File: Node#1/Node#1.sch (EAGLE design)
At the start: 197 parts, among them J1 1757242, J2 DCJ200-10-A-XX-X_REVA, K1 FTR-K1CK005W, K2 FTR-K1CK005W, K3 FTR-K1CK005W, K4 FTR-K1CK005W, U10 ULN2003AIDG4, U11 BLUENRG-232, U12 ACS723LLCTR-40AB-T, U13 RV8564C3, U14 ACS723LLCTR-40AB-T, U2 SEMTECH_SX1503I091TRTSEMTECH_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, U3 MIC4468YWM, U4 LM339ADR, U5 74HC08D,652, U6 SN74LVC1G74DCUR, U7 TMP75BID, U8 IRM-05-5, U9 LMS8117AMP-3.3, X1 2081-1228, X2 2081-1228, X3 2081-1228, X4 2081-1222, Y3 ECS-160-12-36-AGN-TR, Y4 NX2012SA-32.768K-STD-MUB-1

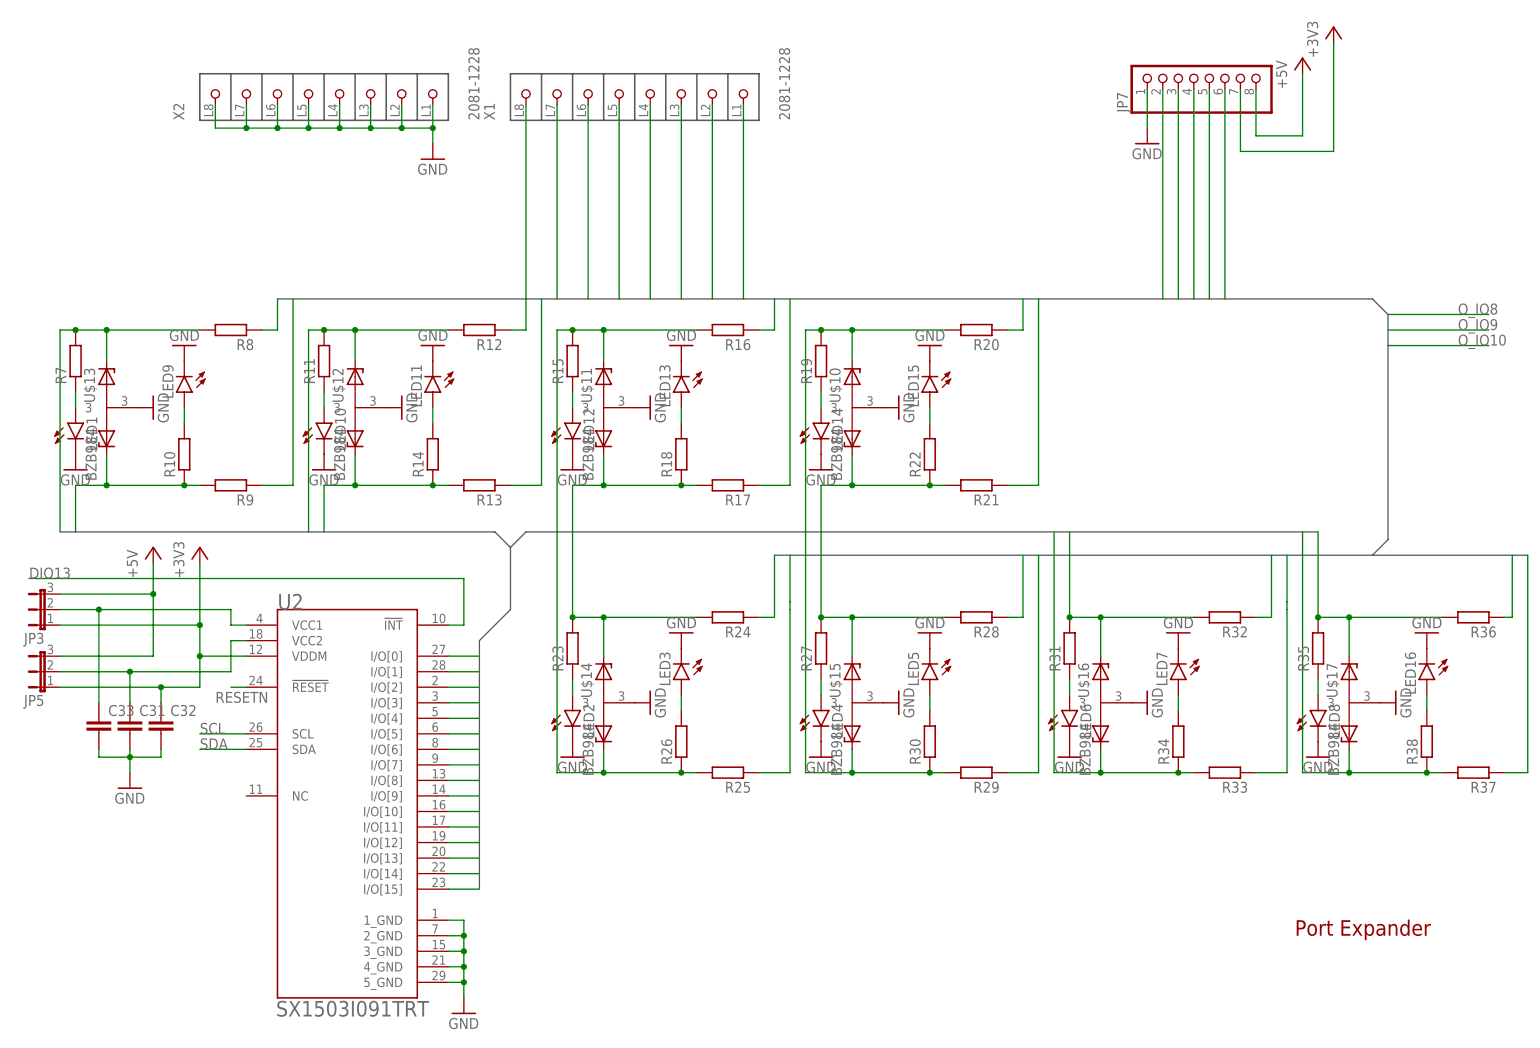
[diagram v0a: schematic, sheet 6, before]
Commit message: Redone Node#1 Layout
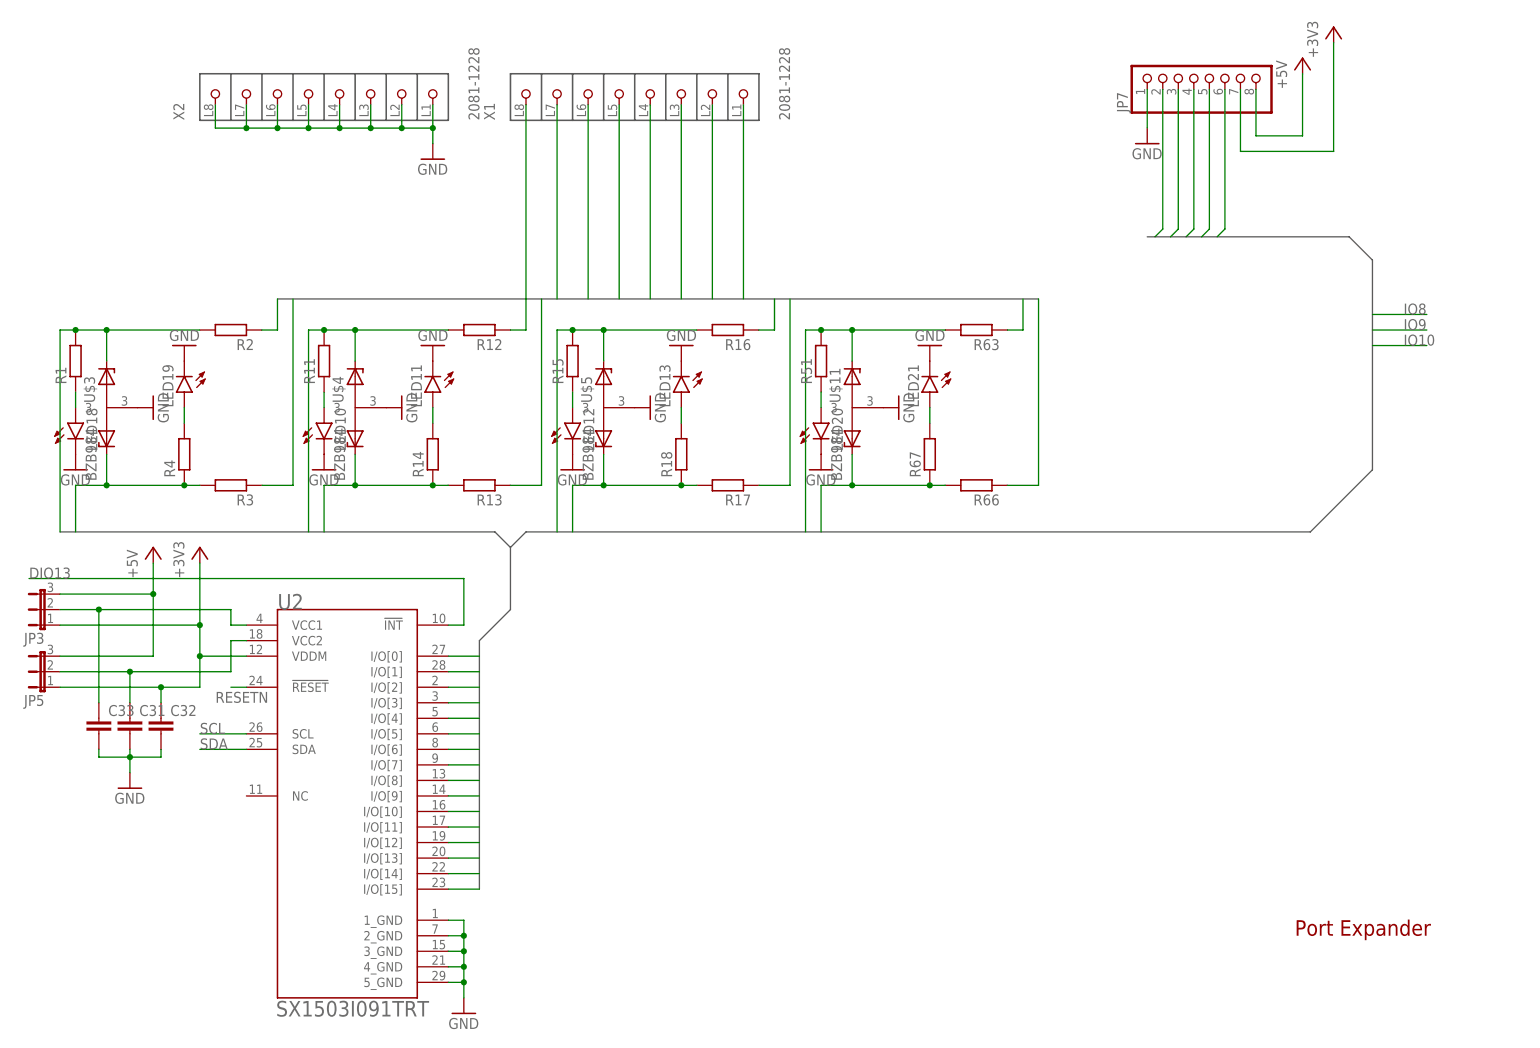
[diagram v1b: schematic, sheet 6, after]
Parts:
- removed LED16, LED2, LED3, LED4, LED5, LED6, LED7, LED8: (no value), led:LED3MM
- removed R23, R24, R25, R26, R27, R28, R29, R30, R31, R32, R33, R34, R35, R36, R37, R38: (no value), rcl:R-EU_R0805
- removed U$10, U$14, U$15, U$16, U$17: BZB984, BlueHome:BZB984
- added U$5: BZB984, BlueHome:BZB984
- renumbered LED1 to LED18, LED14 to LED20, LED15 to LED21, LED9 to LED19, R10 to R4, R19 to R51, R20 to R63, R21 to R66, R22 to R67, R7 to R1, R8 to R2, R9 to R3, U$12 to U$4, U$13 to U$3
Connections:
- removed net E_SHORT: U5.4B, U6.Q
- removed net E_TEMP: R50.1, U5.4A, U7.ALERT
- removed net N$54: LED2.A, R23.1
- removed net N$58: LED3.A, R26.2
- removed net N$60: LED4.A, R27.1
- removed net N$62: LED5.A, R30.2
- removed net N$64: LED6.A, R31.1
- removed net N$66: LED7.A, R34.2
- removed net N$69: LED8.A, R35.1
- removed net N$72: LED16.A, R38.2
- removed net O_IO10: R28.1
- removed net O_IO11: JP7.2, R29.1, R32.1
- removed net O_IO12: JP7.3, R33.1
- removed net O_IO13: JP7.4, R36.1
- removed net O_IO14: JP7.5, R37.1
- removed net O_IO15: JP7.6
- removed net O_IO8: R24.1
- removed net O_IO9: R25.1
- net ERROR: no longer R49.1, U5.4Y
- net GND: now also U$5.3; no longer LED16.C, LED2.C, LED3.C, LED4.C, LED5.C, LED6.C, LED7.C, LED8.C, U$10.3, U$14.3, U$15.3, U$16.3, U$17.3
- net IO10: now also R50.1, U5.4A, U7.ALERT; no longer R27.2, R28.2, U$15.1
- net IO11: now also JP7.2; no longer R29.2, R30.1, U$15.2
- net IO12: now also JP7.3; no longer R31.2, R32.2, U$16.1
- net IO13: now also JP7.4; no longer R33.2, R34.1, U$16.2
- net IO14: now also JP7.5; no longer R35.2, R36.2, U$17.1
- net IO15: now also JP7.6; no longer R37.2, R38.1, U$17.2
- net IO4: now also U$5.1; no longer U$11.1
- net IO5: now also U$5.2; no longer U$11.2
- net IO6: now also U$11.1; no longer U$10.1
- net IO7: now also U$11.2; no longer U$10.2
- net IO8: now also R49.1, U5.4Y; no longer R23.2, R24.2, U$14.1
- net IO9: now also U5.4B, U6.Q; no longer R25.2, R26.1, U$14.2
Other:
- moved on the sheet: U$11

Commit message: Arrangement of Node#1 - DC Power Jack
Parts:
- R53: device rcl:R-EU_R1210 -> rcl:R-EU_R0805
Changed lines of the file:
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@@
 <grid distance="0.1" unitdist="inch" unit="inch" style="lines" multiple="1" display="no" altdistance="0.01" altunitdist="inch" altunit="inch"/>
 <layers>
-<layer number="1" name="Top" color="4" fill="1" visible="no" active="no"/>
-<layer number="2" name="Route2" color="16" fill="1" visible="no" active="no"/>
-<layer number="3" name="Route3" color="17" fill="1" visible="no" active="no"/>
-<layer number="4" name="Route4" color="18" fill="1" visible="no" active="no"/>
-<layer number="5" name="Route5" color="19" fill="1" visible="no" active="no"/>
-<layer number="6" name="Route6" color="25" fill="1" visible="no" active="no"/>
-<layer number="7" name="Route7" color="26" fill="1" visible="no" active="no"/>
-<layer number="8" name="Route8" color="27" fill="1" visible="no" active="no"/>
-<layer number="9" name="Route9" color="28" fill="1" visible="no" active="no"/>
-<layer number="10" name="Route10" color="29" fill="1" visible="no" active="no"/>
-<layer number="11" name="Route11" color="30" fill="1" visible="no" active="no"/>
-<layer number="12" name="Route12" color="20" fill="1" visible="no" active="no"/>
-<layer number="13" name="Route13" color="21" fill="1" visible="no" active="no"/>
-<layer number="14" name="Route14" color="22" fill="1" visible="no" active="no"/>
-<layer number="15" name="Route15" color="23" fill="1" visible="no" active="no"/>
-<layer number="16" name="Bottom" color="1" fill="1" visible="no" active="no"/>
-<layer number="17" name="Pads" color="2" fill="1" visible="no" active="no"/>
-<layer number="18" name="Vias" color="2" fill="1" visible="no" active="no"/>
-<layer number="19" name="Unrouted" color="6" fill="1" visible="no" active="no"/>
-<layer number="20" name="Dimension" color="24" fill="1" visible="no" active="no"/>
-<layer number="21" name="tPlace" color="7" fill="1" visible="no" active="no"/>
-<layer number="22" name="bPlace" color="7" fill="1" visible="no" active="no"/>
-<layer number="23" name="tOrigins" color="15" fill="1" visible="no" active="no"/>
-<layer number="24" name="bOrigins" color="15" fill="1" visible="no" active="no"/>
-<layer number="25" name="tNames" color="7" fill="1" visible="no" active="no"/>
-<layer number="26" name="bNames" color="7" fill="1" visible="no" active="no"/>
-<layer number="27" name="tValues" color="7" fill="1" visible="no" active="no"/>
-<layer number="28" name="bValues" color="7" fill="1" visible="no" active="no"/>
+<layer number="1" name="Top" color="4" fill="1" visible="yes" active="no"/>
+<layer number="2" name="Route2" color="16" fill="1" visible="yes" active="no"/>
+<layer number="3" name="Route3" color="17" fill="1" visible="yes" active="no"/>
+<layer number="4" name="Route4" color="18" fill="1" visible="yes" active="no"/>
+<layer number="5" name="Route5" color="19" fill="1" visible="yes" active="no"/>
+<layer number="6" name="Route6" color="25" fill="1" visible="yes" active="no"/>
+<layer number="7" name="Route7" color="26" fill="1" visible="yes" active="no"/>
+<layer number="8" name="Route8" color="27" fill="1" visible="yes" active="no"/>
+<layer number="9" name="Route9" color="28" fill="1" visible="yes" active="no"/>
+<layer number="10" name="Route10" color="29" fill="1" visible="yes" active="no"/>
+<layer number="11" name="Route11" color="30" fill="1" visible="yes" active="no"/>
+<layer number="12" name="Route12" color="20" fill="1" visible="yes" active="no"/>
+<layer number="13" name="Route13" color="21" fill="1" visible="yes" active="no"/>
+<layer number="14" name="Route14" color="22" fill="1" visible="yes" active="no"/>
+<layer number="15" name="Route15" color="23" fill="1" visible="yes" active="no"/>
+<layer number="16" name="Bottom" color="1" fill="1" visible="yes" active="no"/>
+<layer number="17" name="Pads" color="2" fill="1" visible="yes" active="no"/>
+<layer number="18" name="Vias" color="2" fill="1" visible="yes" active="no"/>
+<layer number="19" name="Unrouted" color="6" fill="1" visible="yes" active="no"/>
+<layer number="20" name="Dimension" color="24" fill="1" visible="yes" active="no"/>
+<layer number="21" name="tPlace" color="7" fill="1" visible="yes" active="no"/>
+<layer number="22" name="bPlace" color="7" fill="1" visible="yes" active="no"/>
+<layer number="23" name="tOrigins" color="15" fill="1" visible="yes" active="no"/>
+<layer number="24" name="bOrigins" color="15" fill="1" visible="yes" active="no"/>
+<layer number="25" name="tNames" color="7" fill="1" visible="yes" active="no"/>
+<layer number="26" name="bNames" color="7" fill="1" visible="yes" active="no"/>
+<layer number="27" name="tValues" color="7" fill="1" visible="yes" active="no"/>
+<layer number="28" name="bValues" color="7" fill="1" visible="yes" active="no"/>
 <layer number="29" name="tStop" color="7" fill="3" visible="no" active="no"/>
 <layer number="30" name="bStop" color="7" fill="6" visible="no" active="no"/>
@@
 <layer number="35" name="tGlue" color="7" fill="4" visible="no" active="no"/>
 <layer number="36" name="bGlue" color="7" fill="5" visible="no" active="no"/>
-<layer number="37" name="tTest" color="7" fill="1" visible="no" active="no"/>
-<layer number="38" name="bTest" color="7" fill="1" visible="no" active="no"/>
+<layer number="37" name="tTest" color="7" fill="1" visible="yes" active="no"/>
+<layer number="38" name="bTest" color="7" fill="1" visible="yes" active="no"/>
 <layer number="39" name="tKeepout" color="4" fill="11" visible="no" active="no"/>
 <layer number="40" name="bKeepout" color="1" fill="11" visible="no" active="no"/>
@@
 <layer number="44" name="Drills" color="7" fill="1" visible="no" active="no"/>
 <layer number="45" name="Holes" color="7" fill="1" visible="no" active="no"/>
-<layer number="46" name="Milling" color="3" fill="1" visible="no" active="no"/>
-<layer number="47" name="Measures" color="7" fill="1" visible="no" active="no"/>
-<layer number="48" name="Document" color="7" fill="1" visible="no" active="no"/>
-<layer number="49" name="Reference" color="7" fill="1" visible="no" active="no"/>
-<layer number="51" name="tDocu" color="7" fill="1" visible="no" active="no"/>
-<layer number="52" name="bDocu" color="7" fill="1" visible="no" active="no"/>
+<layer number="46" name="Milling" color="3" fill="1" visible="yes" active="no"/>
+<layer number="47" name="Measures" color="7" fill="1" visible="yes" active="no"/>
+<layer number="48" name="Document" color="7" fill="1" visible="yes" active="no"/>
+<layer number="49" name="Reference" color="7" fill="1" visible="yes" active="no"/>
+<layer number="51" name="tDocu" color="7" fill="1" visible="yes" active="no"/>
+<layer number="52" name="bDocu" color="7" fill="1" visible="yes" active="no"/>
 <layer number="88" name="SimResults" color="9" fill="1" visible="no" active="yes"/>
 <layer number="89" name="SimProbes" color="9" fill="1" visible="no" active="yes"/>
@@
 <part name="J2" library="BlueHome" deviceset="DCJ200-10-A-XX-X_REVA" device=""/>
 <part name="X4" library="BlueHome" deviceset="2081-1222" device=""/>
-<part name="R53" library="rcl" library_urn="urn:adsk.eagle:library:334" deviceset="R-EU_" device="R1210" package3d_urn="urn:adsk.eagle:package:23554/2"/>
+<part name="R53" library="rcl" library_urn="urn:adsk.eagle:library:334" deviceset="R-EU_" device="R0805" package3d_urn="urn:adsk.eagle:package:23553/2"/>
 <part name="+3V16" library="supply1" library_urn="urn:adsk.eagle:library:371" deviceset="+3V3" device=""/>
 <part name="P+6" library="supply1" library_urn="urn:adsk.eagle:library:371" deviceset="+5V" device=""/>
